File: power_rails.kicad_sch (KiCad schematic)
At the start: 24 parts, among them SW3 SW_Push, U10 LTC2954CDDB-1-PBF, U5 AP63200WU, U7 AP63205WU, U9 TPS62162DSG

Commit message: tentative automatic population
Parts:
- C13, C19: LCSC (none) -> C14663; MPN (none) -> CC0603KRX7R9BB104; Manufacturer (none) -> YAGEO
- C17, C20, C21, C23, C24, C28: LCSC (none) -> C296720; MPN (none) -> CL21A226KOQNNNE; Manufacturer (none) -> Samsung Electro-Mechanics
- C18, C22, C25: LCSC (none) -> C84416; MPN (none) -> GRM21BR61E106KA73L; Manufacturer (none) -> muRata
- C26: LCSC (none) -> C29266; MPN (none) -> CL05A105KO5NNNC; Manufacturer (none) -> Samsung Electro-Mechanics
- D3: LCSC (none) -> C2286; MPN (none) -> KT-0603R; Manufacturer (none) -> Hubei KENTO Elec
- L2: LCSC (none) -> C2844756; MPN (none) -> LPS3015-222MRC; Manufacturer (none) -> Coilcraft
- L3: LCSC (none) -> C108284; MPN (none) -> LVS505040-4R7M-N; Manufacturer (none) -> Chilisin
- L4: LCSC (none) -> C431344; MPN (none) -> CMLW5040S100MST; Manufacturer (none) -> Cybermax
- R11: LCSC (none) -> C14891; MPN (none) -> 0603WAF6492T5E; Manufacturer (none) -> UNI-ROYAL
- R12: LCSC (none) -> C2906982; MPN (none) -> FRC0603F1002TS; Manufacturer (none) -> FOJAN
- R15: LCSC (none) -> C25803; MPN (none) -> 0603WAF1003T5E; Manufacturer (none) -> UNI-ROYAL
- SW3: LCSC (none) -> C231329; MPN (none) -> B3U-1000P; Manufacturer (none) -> OMRON
- U5: LCSC (none) -> C2071868; MPN (none) -> AP63200WU-7; Manufacturer (none) -> DIODES
- U7: LCSC (none) -> C2071056; MPN (none) -> AP63205WU-7; Manufacturer (none) -> DIODES
- U9: LCSC (none) -> C40256; MPN (none) -> TPS62162DSGR; Manufacturer (none) -> TI

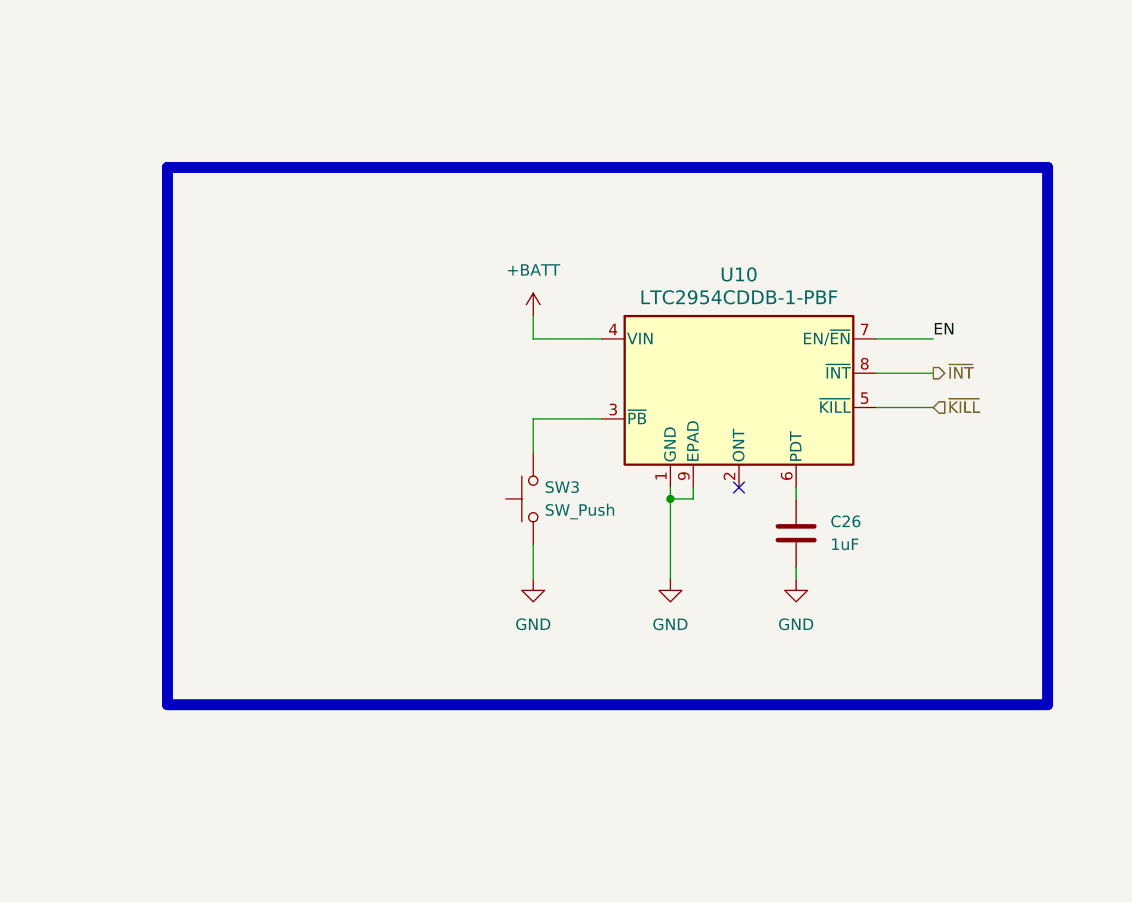
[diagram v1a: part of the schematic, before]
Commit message: Consistent final layout
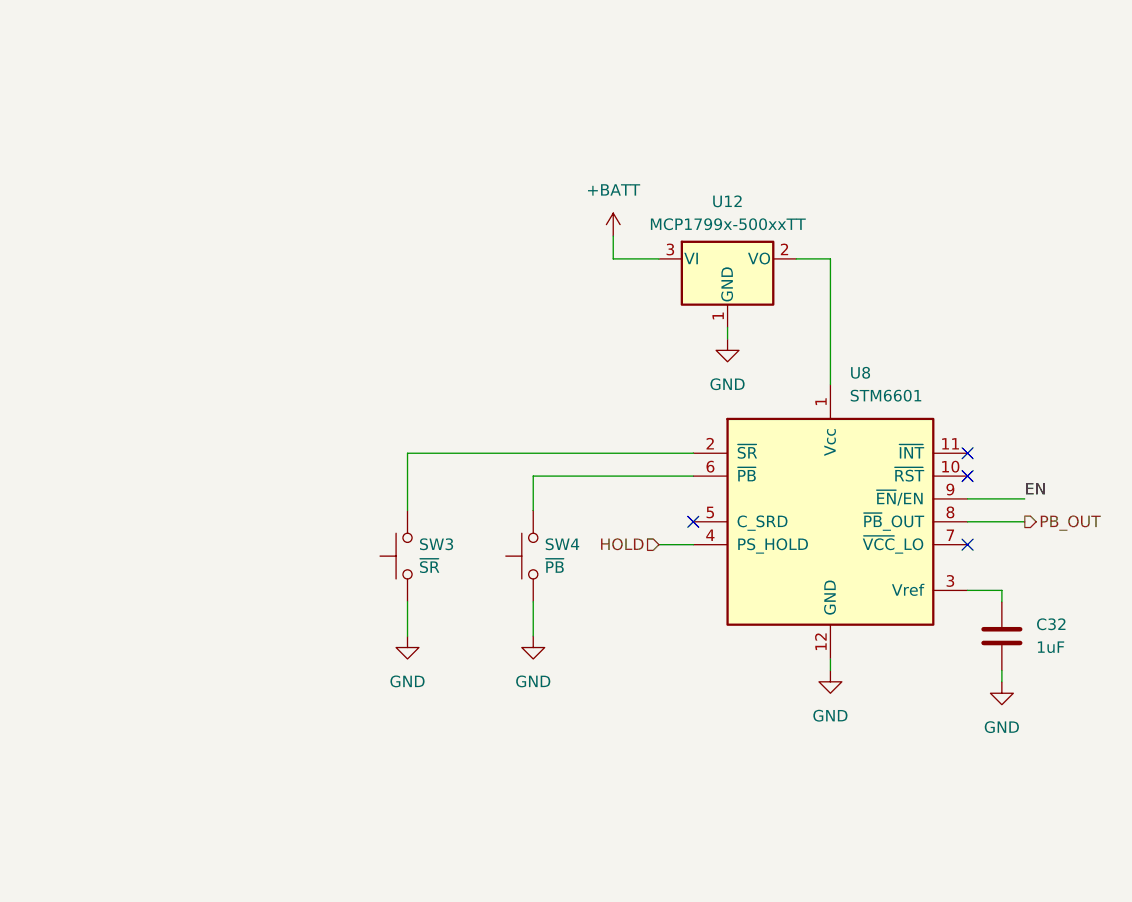
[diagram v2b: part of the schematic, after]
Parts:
- removed C26: 1uF, Capacitor_SMD:C_0402_1005Metric, symbol Device:C
- removed U10: LTC2954CDDB-1-PBF, Package_DFN_QFN:DFN-8-1EP_2x3mm_P0.5mm_EP0.61x2.2mm, symbol LTC2954CDDB:LTC2954CDDB-1-PBF
- added C32: 1uF, Capacitor_SMD:C_0603_1608Metric, symbol Device:C
- added SW4: ~{PB}, Button_Switch_SMD:SW_SPST_B3U-1000P, symbol Switch:SW_Push
- added U12: MCP1799x-500xxTT, Package_TO_SOT_SMD:SOT-23, symbol Regulator_Linear:MCP1799x-500xxTT
- added U8: STM6601, Package_DFN_QFN:TDFN-12_2x3mm_P0.5mm, symbol Power_Management:STM6601
- SW3: value SW_Push -> ~{SR}
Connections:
- net +BATT: now also U12.3 (VI)
- net EN: now also U8.9 (~{EN}/EN)
- net GND: now also C32.2, SW4.1, U12.1 (GND), U8.12 (GND)
- net at SW3.2: now also U8.2 (~{SR})
- new net: U12.2 (VO), U8.1 (Vcc)
- new net: SW4.2, U8.6 (~{PB})
- new net: C32.1, U8.3 (Vref)
- new net HOLD: U8.4 (PS_HOLD)
- new net PB_OUT: U8.8 (~{PB}_OUT)
- no-connect marks 1 -> 4
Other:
- moved on the sheet: SW3
